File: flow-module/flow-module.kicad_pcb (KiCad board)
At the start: 2 copper layers, 60 x 47.2 mm, 22 parts, among them P1 12V, P2 tL298P, P3 tLMD..., P4 fL298P, P5 fLMD...

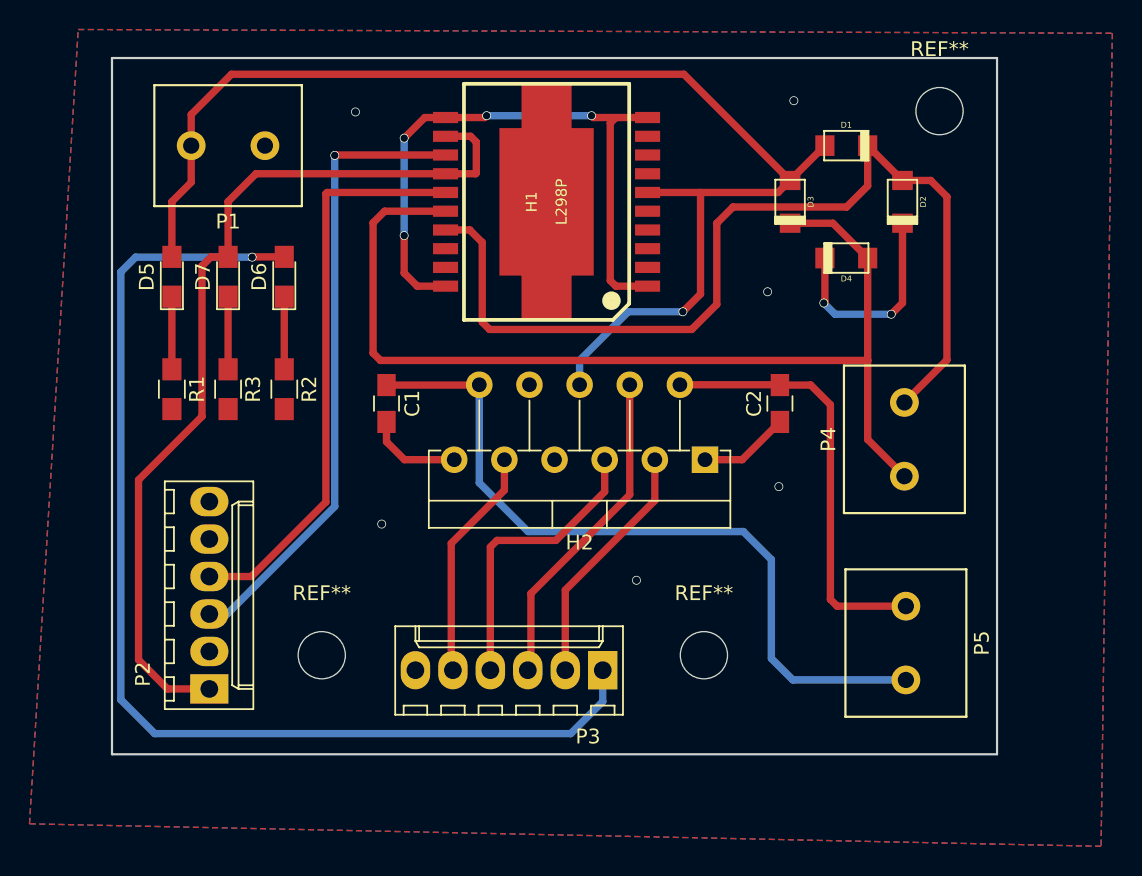
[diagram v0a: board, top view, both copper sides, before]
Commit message: PCB Design update
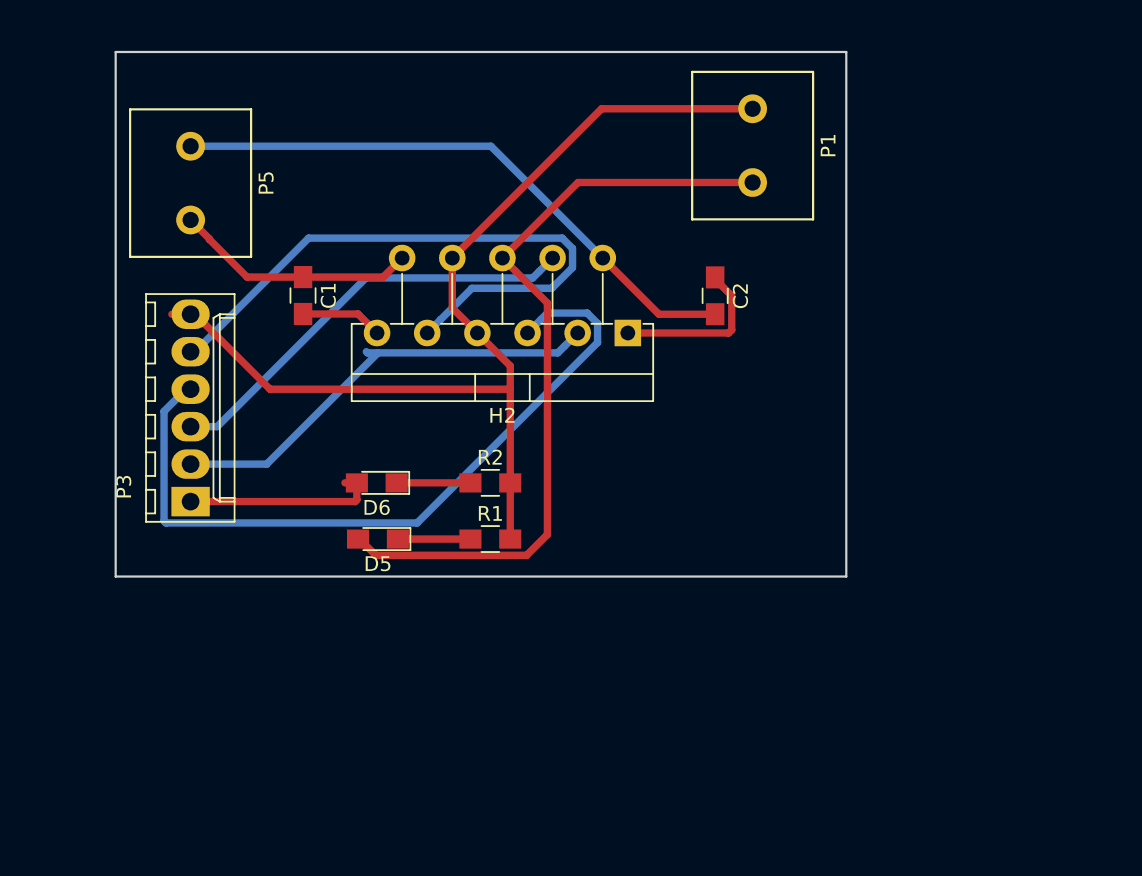
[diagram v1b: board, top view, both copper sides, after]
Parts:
- removed D1, D2, D3, D4: D, ValveTeam:do219ab
- removed D7: VSS, LEDs:LED_0805_HandSoldering
- removed H1: L298P, ValveTeam:powerso-20
- removed P2: tL298P, ValveTeam:Molex_KK-6410-06_06x2.54mm_Straight
- removed P4: fL298P, ValveTeam:TE_TERM
- removed R3: 330, Resistors_SMD:R_0805_HandSoldering
- removed REF** (x3): MountingHole_3.2mm_M3, Mounting_Holes:MountingHole_3.2mm_M3
- D5: value VCC -> LED
- D6: value VAA -> LED
- P1: value 12V -> TERM_01X02
- P3: value tLMD... -> MOLEX_01X06
- P5: value fLMD... -> TERM_01X02
- moved P5 57.6 mm to (74.9, 30.5)
- moved P1 35.6 mm to (113.0, 27.9), turned to 90 degrees
- moved P3 30.2 mm to (74.9, 52.1), turned to 90 degrees
- moved R1 23.9 mm to (95.2, 54.6), turned to 0 degrees
- moved D5 22.6 mm to (87.6, 54.6), turned to 180 degrees
- moved R2 15.3 mm to (95.2, 50.8), turned to 0 degrees
- moved D6 15.3 mm to (87.5, 50.8), turned to 180 degrees
- moved H2 10.1 mm to (104.6, 40.6)
- moved C1 9.25 mm to (82.5, 38.1)
- moved C2 8.52 mm to (110.5, 38.1), turned to 270 degrees
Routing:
- net Net-(D3-Pad2): track 69.9 -> 0.00 mm
- net Net-(D1-Pad2): track 66.5 -> 0.00 mm
- net VAA: track 77.2 -> 13.3 mm, vias 1 -> 0
- net VSS: track 61.9 -> 0.00 mm
- net Input3: track 42.8 -> 0.00 mm, vias 1 -> 0
- net Input4: track 39.0 -> 0.00 mm
- net Output2: track 51.3 -> 16.5 mm
- net VCC: track 86.8 -> 53.0 mm, vias 1 -> 0
- net PWM: track 19.8 -> 51.3 mm
- net Flag: track 15.8 -> 42.4 mm
- net Dir: track 16.8 -> 30.7 mm
- net Earth: track 57.8 -> 69.3 mm, vias 6 -> 0
- net Output1: track 29.3 -> 40.3 mm
- net Brake: track 22.2 -> 29.3 mm
- net Net-(C2-Pad1): track 6.14 -> 11.2 mm
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- removed copper zone on B.Cu, net Earth
- removed copper zone on F.Cu, net Earth
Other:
- board size 60 x 47.2 mm -> 49.5 x 35.6 mm
